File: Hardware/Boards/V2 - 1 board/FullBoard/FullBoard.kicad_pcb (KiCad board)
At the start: 2 copper layers, 145.3 x 73.4 mm, 28 parts, among them J1 Conn_01x03_Pin, J2 Conn_01x03_Pin, J3 Conn_01x02_Pin, J4 Conn_01x03_Pin, J5 Conn_01x03_Pin, J6 Conn_01x02_Pin, U1 GY-8511 UV sensor, U2 TEMT6000, U3 DS18B20-air, U4 Turbidity sensor, U5 DS18B20-water, U6 Water Level Sensor, U7 ESP32, U8 Relay module

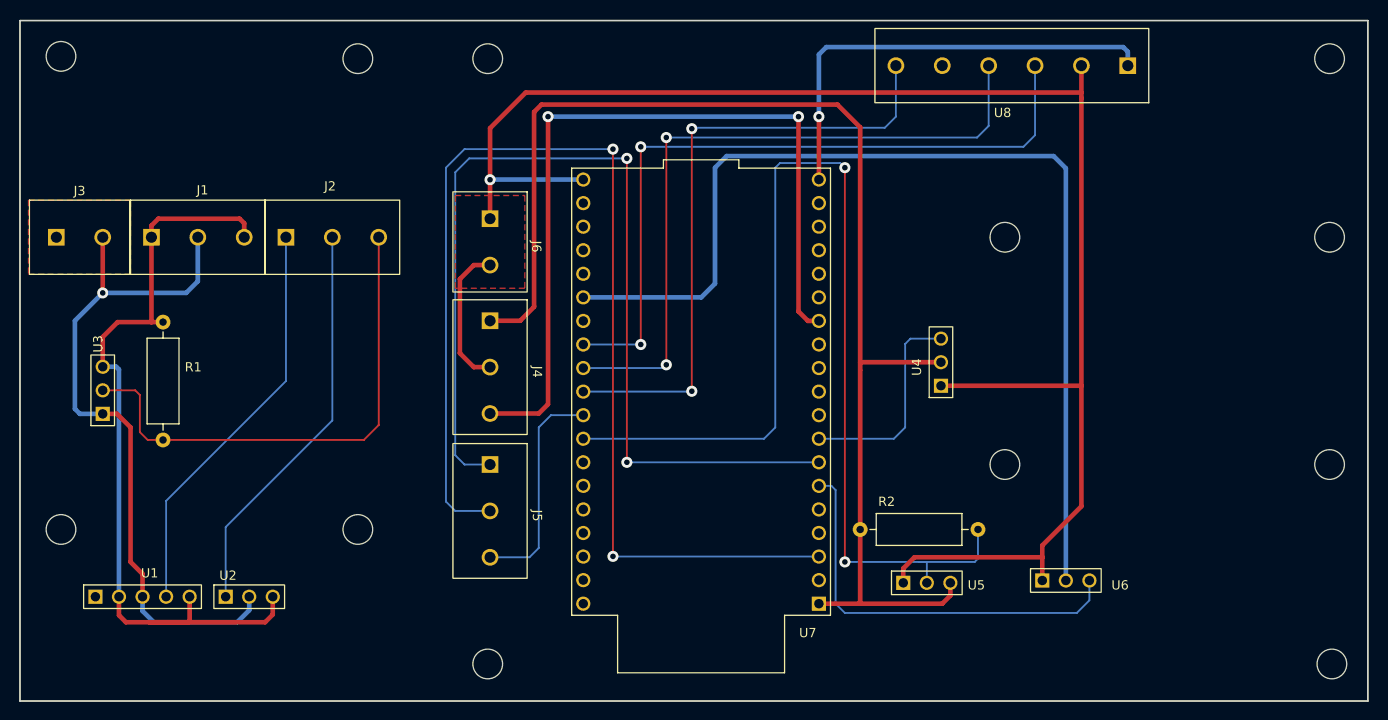
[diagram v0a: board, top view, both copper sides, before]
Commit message: PCB almost complete
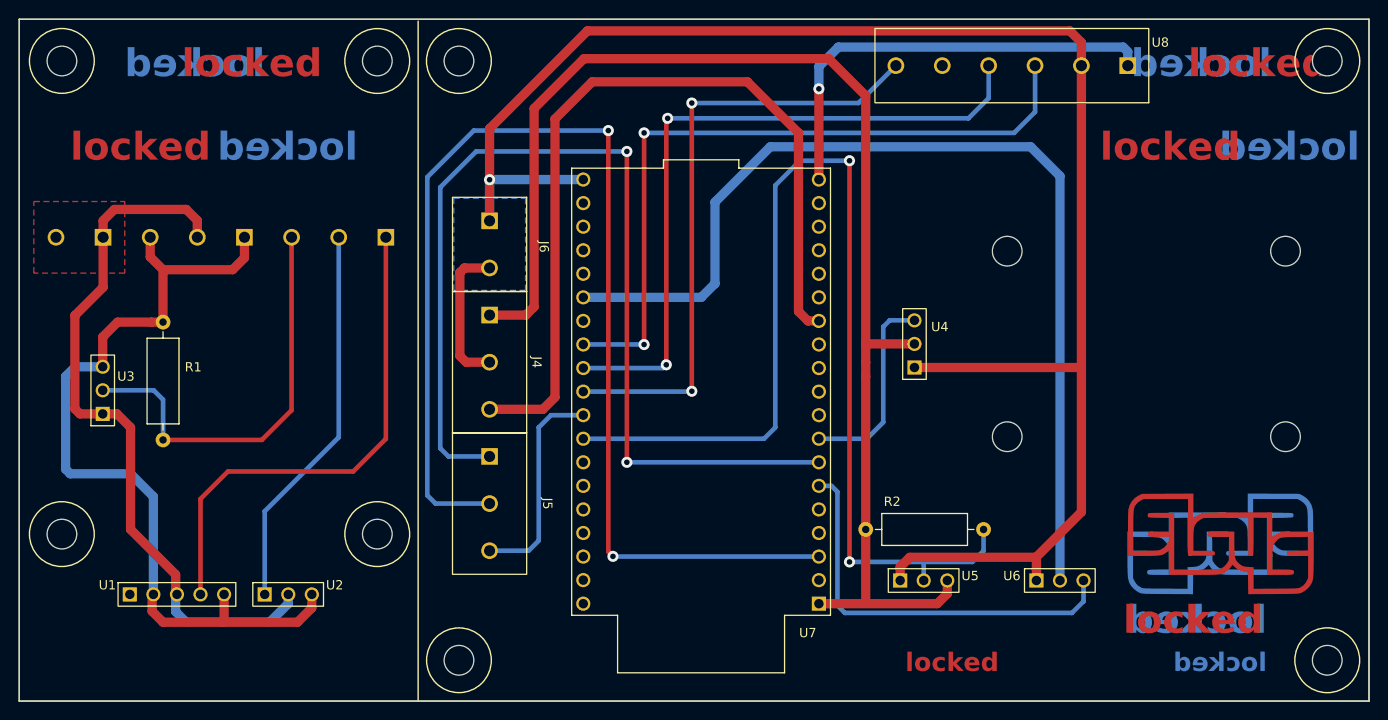
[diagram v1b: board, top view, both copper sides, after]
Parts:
- added G***: LOGO, LOGO, F.Cu at (180.0, 97.0)
- added G***: LOGO, LOGO, B.Cu at (180.0, 97.0)
- J1, J2, J3: moved to B.Cu
- U3, U5: footprint Diplomna:DS18B20_3dmodel -> Diplomna:3pin_holes
- moved U1 8.79 mm to (67.5, 102.5)
- moved U6 6.25 mm to (162.7, 101.0)
- moved U4 6.23 mm to (147.0, 75.5)
- moved U5 6.09 mm to (148.0, 101.0)
- moved U3 5.68 mm to (59.5, 80.5)
- moved REF** 5.62 mm to (187.0, 85.5)
- moved REF** 4.98 mm to (187.0, 65.5)
- moved REF** 3.13 mm to (97.9, 109.6)
- moved REF** 3.11 mm to (97.9, 45.0)
- moved REF** 3.01 mm to (157.0, 85.5)
- moved U2 2.92 mm to (79.5, 102.5)
- moved REF** 2.16 mm to (89.1, 96.0)
- moved REF** 2.11 mm to (89.1, 45.0)
- moved REF** 1.52 mm to (157.0, 65.5)
- moved J5 1.29 mm to (101.2, 92.7)
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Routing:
- net GND: track 190.3 -> 203.7 mm
- net /uv_out: track 44.1 -> 54.7 mm
- net /air_temp: track 55.2 -> 45.1 mm
- net /brightness_out_main: track 126.1 -> 131.3 mm
- net +3V3: track 87.4 -> 91.8 mm
- net +3.3V: track 138.9 -> 141.7 mm
- net /uv_out_main: track 107.3 -> 109.8 mm
- net /water_level_power: track 110.6 -> 108.2 mm
- net /brightness_out: track 43.5 -> 41.8 mm
- net /relay_heater: track 68.1 -> 66.5 mm
- net /water_temp: track 120.4 -> 118.9 mm
- net /uv_ref_main: track 88.3 -> 89.7 mm, vias 2 -> 0
- net /turbidity: track 22.9 -> 21.6 mm
- net GND1: track 76.4 -> 77.6 mm, vias 1 -> 0
- net +5V: track 48.8 -> 48.1 mm
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- added copper zone on B.Cu, net GND
- removed copper zone on F.Cu, net GND
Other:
- board size 145.3 x 73.4 mm -> 145.5 x 73.5 mm
- board text added: "locked"
